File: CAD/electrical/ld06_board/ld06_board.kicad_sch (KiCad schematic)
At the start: 15 parts, among them J1 SERIAL, J2 LED Strip, J3 Conn_01x02_Pin, J4 I2C, J5 Conn_01x02_Pin, J6 Conn_01x02_Pin, J7 I2C, J9 Battery in, U1 TXBN0304RUT, U2 SeeeduinoXIAO, U3 LM7805_TO220

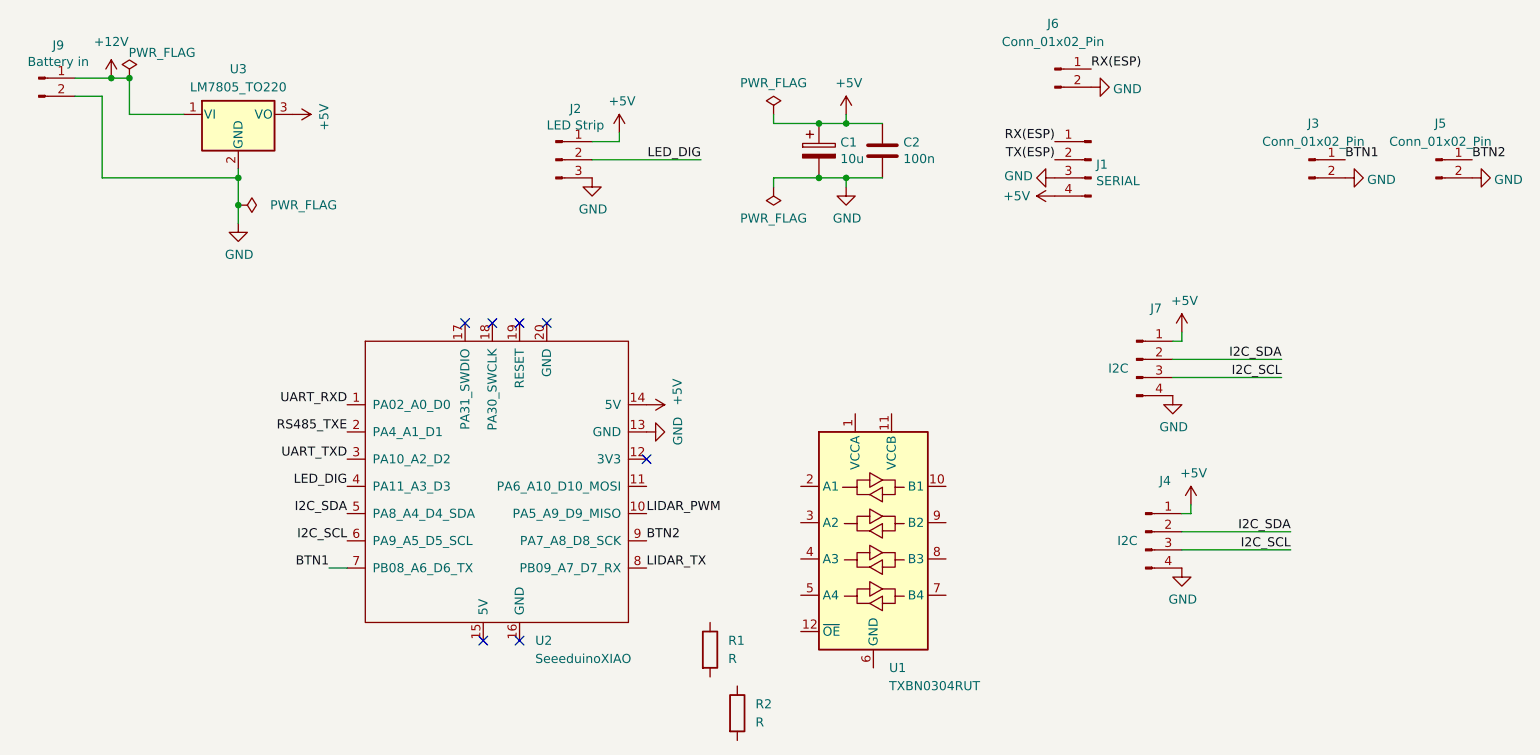
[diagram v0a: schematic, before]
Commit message: update
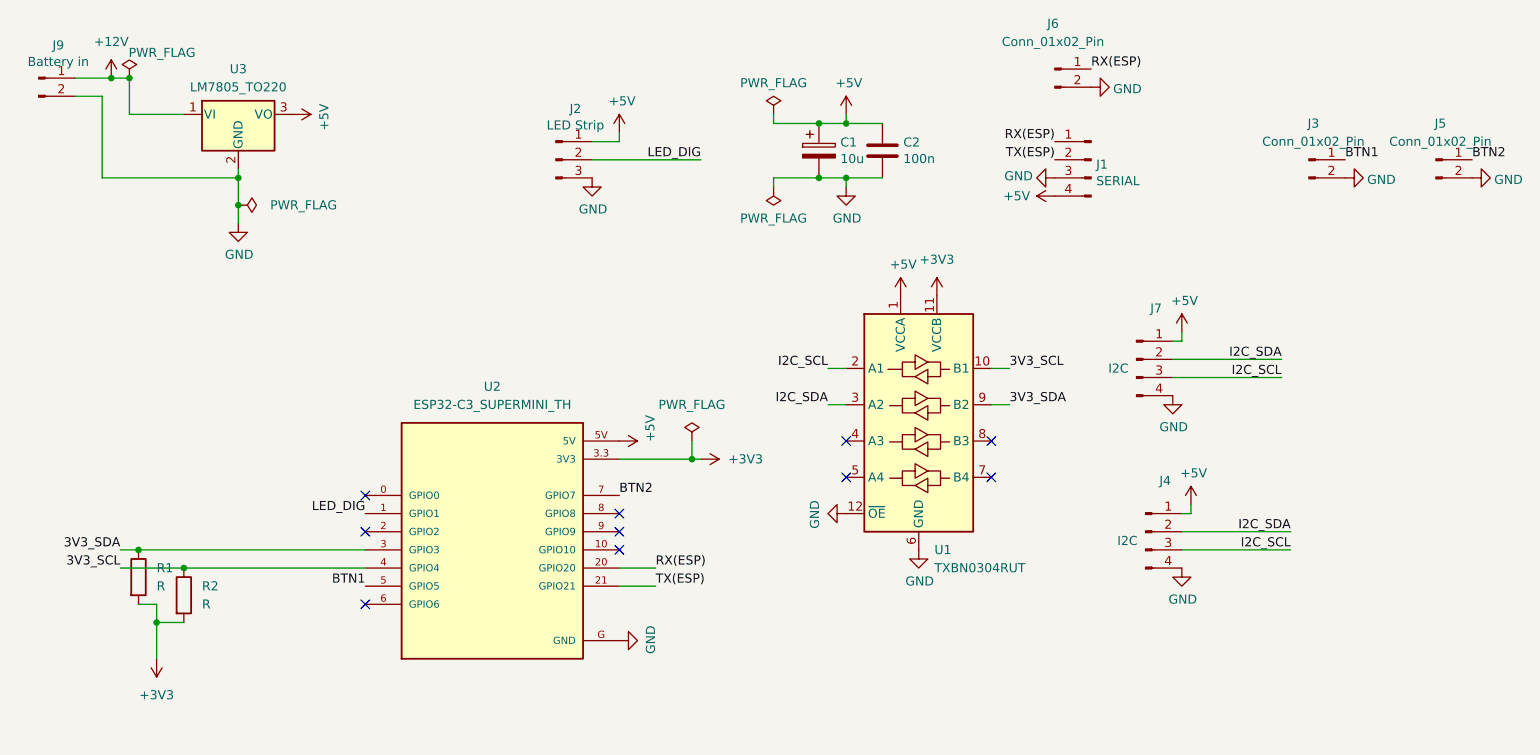
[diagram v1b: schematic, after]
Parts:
- removed U2: SeeeduinoXIAO, Seeeduino XIAO KICAD:XIAO-ESP32-C3-DIP, symbol Seeeduino XIAO:SeeeduinoXIAO
- added U2: ESP32-C3_SUPERMINI_TH, ESP32-C3_SUPERMINI_TH:MODULE_ESP32-C3_SUPERMINI, symbol ESP32-C3_SUPERMINI_TH:ESP32-C3_SUPERMINI_TH
- U1: footprint Package_DIP:DIP-12_W10.16mm -> (none)
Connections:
- net +5V: now also U1.1 (VCCA), U2.5V
- net BTN1: now also U2.5 (GPIO5)
- net BTN2: now also U2.7 (GPIO7)
- net GND: now also U1.12 (~{OE}), U1.6 (GND), U2.G (GND)
- net I2C_SCL: now also U1.2 (A1)
- net I2C_SDA: now also U1.3 (A2)
- net LED_DIG: now also U2.1 (GPIO1)
- net RX(ESP): now also U2.20 (GPIO20)
- net TX(ESP): now also U2.21 (GPIO21)
- net 3V3_SCL: now reaches R2.1
- net 3V3_SCL: now also U1.10 (B1), U2.4 (GPIO4)
- net +3V3: now reaches R2.2
- net +3V3: now also R1.2, U1.11 (VCCB), U2.3.3 (3V3)
- net 3V3_SDA: now reaches R1.1
- net 3V3_SDA: now also U1.9 (B2), U2.3 (GPIO3)
- no-connect marks 7 -> 10
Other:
- moved on the sheet: U1
